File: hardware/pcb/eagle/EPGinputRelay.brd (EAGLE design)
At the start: 45 x 22 mm, 28 parts, among them J1 54-00248, U1 ADA4530-1, U2 ADA4530-1, U3 ADA4940-1

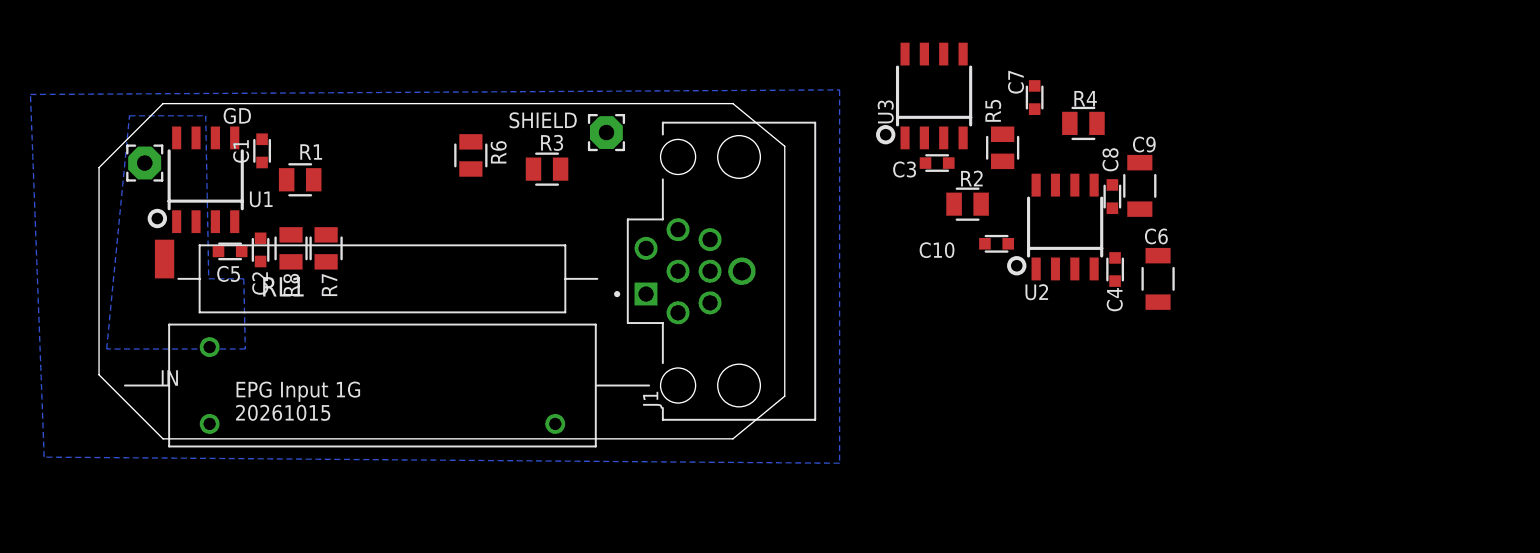
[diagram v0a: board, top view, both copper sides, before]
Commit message: PCB w/ relay
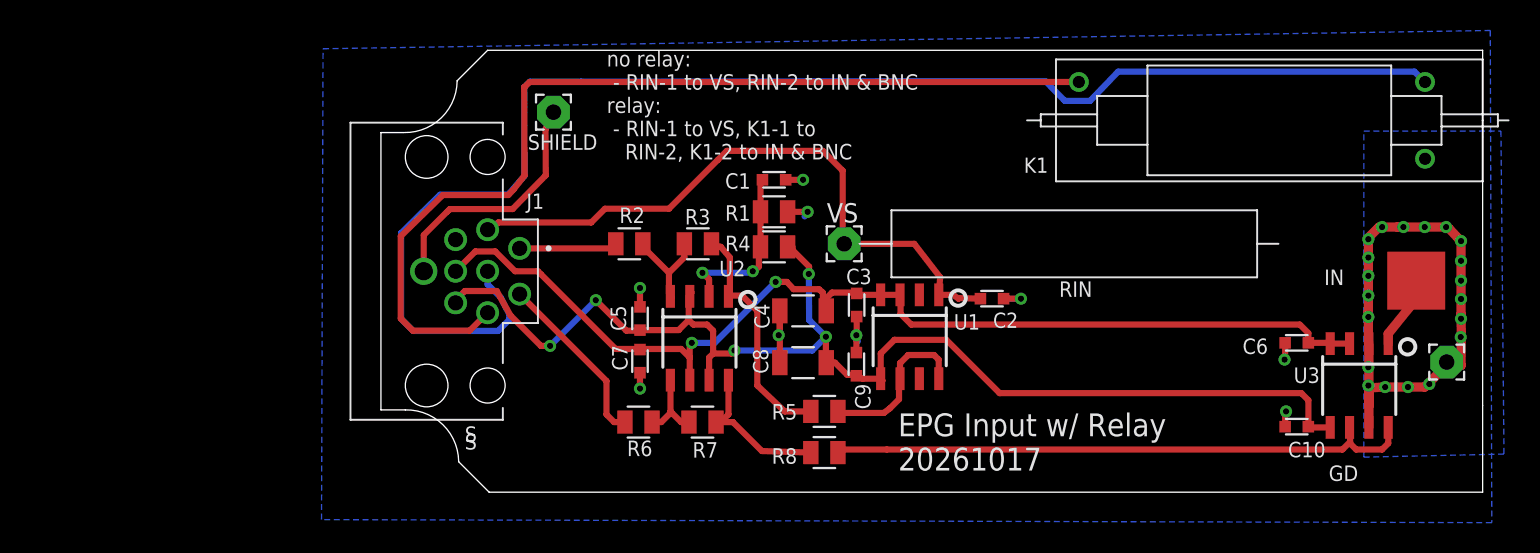
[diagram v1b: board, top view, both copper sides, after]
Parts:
- removed RL1: REED-RELAY, EPGinput:MRE05
- removed U$2: (no value), EPGinput:1GRES
- added K1: REED-RELAY, EPGinput:MRE05
- added RIN: (no value), EPGinput:1GRES
- added VS: (no value), wirepad:2,15/1,0
- C10: value 0.1 -> (none)
- C2: value (none) -> 0.1
- C4, C8: value (none) -> 10; device STEVES_BU:0603S -> STEVES_BU:1206S
- C6, C9: value 10 -> (none); device STEVES_BU:1206S -> STEVES_BU:0603S
- IN: device wirepad:SMD1,27-2,54 -> jETPAK-ASM:PAD-150SQ
- U$1: value POMONA2397 -> (none); device STEVES_BU:POMONA2397 -> EPGinput:BNC
- U2: value ADA4530-1 -> ADA4940-1
- U3: value ADA4940-1 -> ADA4530-1
- moved GD 86.4 mm to (69.9, -5.96), turned to 180 degrees
- moved IN 82.2 mm to (67.9, -0.62)
- moved C2 48.1 mm to (40.1, -1.80), turned to 0 degrees
- moved U$1 48.0 mm to (83.8, 0.00)
- moved U1 47.3 mm to (34.7, -4.30), turned to 180 degrees
- moved R8 37.5 mm to (29.1, -11.9), turned to 180 degrees
- moved U3 33.8 mm to (64.2, -7.50), turned to 180 degrees
- moved C1 33.7 mm to (25.8, 6.00), turned to 0 degrees
- moved R1 31.2 mm to (25.8, 3.90), turned to 180 degrees
- moved C7 31.1 mm to (17.0, -5.90)
- moved C5 27.3 mm to (17.0, -3.10), turned to 90 degrees
- moved R7 27.2 mm to (21.1, -9.90), turned to 180 degrees
- moved U2 25.1 mm to (20.9, -4.40), turned to 180 degrees
- moved C10 23.1 mm to (60.1, -10.2)
- moved C8 23.0 mm to (27.7, -6.00), turned to 180 degrees
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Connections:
- removed net N$1: C2.1, R7.1, R8.2, U3.2
- removed net RLY: J1.3, RL1.COIL2
- removed net SHIELD: J1.8, J1.S1, SHIELD.1
- new net N$2: J1.S1, SHIELD.1
- new net RLY+: J1.3, K1.COIL2
- new net RLY-: J1.8, K1.COIL1
- new net VCOM: C1.1, R1.2, R4.1, U2.2
- net -5V0: now also C3.1, U2.6, U3.3, U3.4; no longer C5.1, U2.3, U2.4, U3.6
- net 5V0: now also C10.1, C5.1, C8.1, C9.2, R4.2, U2.3, U2.7, U3.5; no longer C1.1, C3.1, C8.2, C9.1, R7.2, U2.5, U3.3, U3.7
- net GND: now also C8.2, C9.1, R1.1; no longer C8.1, C9.2, R8.1, RL1.COIL1
- net GUARD: now also K1.GUARD, U3.2, U3.7; no longer RL1.GUARD, U1.2, U1.7
- net N$10: now also R2.2; no longer R4.2
- net N$19: now also R2.1, R3.2, U2.4; no longer R4.1, R5.2, U3.4
- net N$20: now also R6.1, R7.2, U2.5; no longer R3.1, R6.2, U3.5
- net N$6: now also R7.1, R8.2, U2.8; no longer R1.2, R6.1, U3.8
- net N$7: now also R3.1, R5.2, U2.1; no longer R2.2, R5.1, U3.1
- net N$9: now also R6.2; no longer R3.2
- net PROBE: now also IN.P$1, U3.1; no longer IN.1, U1.1
- net SIGOUT: now also R8.1, U3.6, U3.8; no longer R1.1, U1.6, U1.8
- net VS: now also C2.1, U1.1, VS.1; no longer C10.1, U2.1
- net VSOUT: now also R5.1, U1.6, U1.8; no longer R2.1, U2.6, U2.8
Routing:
- net RLY-: track 0.00 -> 93.4 mm
- net 5V0: track 0.00 -> 83.0 mm, vias 0 -> 5
- net -5V0: track 0.00 -> 71.2 mm, vias 0 -> 2
- net RLY+: track 0.00 -> 64.1 mm
- net VS: track 0.00 -> 42.2 mm
- net SIGOUT: track 0.00 -> 38.8 mm
- net GUARD: track 0.00 -> 36.8 mm, vias 0 -> 20
- net GND: track 0.00 -> 18.6 mm, vias 0 -> 9
- net N$2: track 0.00 -> 16.3 mm
- net N$7: track 0.00 -> 15.4 mm
- net N$9: track 0.00 -> 11.7 mm
- net VCOM: track 0.00 -> 11.6 mm, vias 0 -> 2
- net VSOUT: track 0.00 -> 10.9 mm
- net N$6: track 0.00 -> 9.97 mm
- net N$19: track 0.00 -> 6.58 mm
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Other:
- board size 45 x 22 mm -> 72.3 x 29 mm
- board text added: "EPG Input w/ Relay 20261017"
- board text added: "S"
- board text added: "no relay: - RIN-1 to VS, RIN-2 to IN & BNC relay: - RIN-1 to VS, K1-1 to RIN-2, K1-2 to IN & BNC"
- board text removed: "EPG Input 1G 20261015"

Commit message: started control board
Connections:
- net N$10 renamed AOP\
- net N$9 renamed AON
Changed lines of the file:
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@@
 <layer number="14" name="Route14" color="1" fill="6" visible="no" active="no"/>
 <layer number="15" name="Route15" color="4" fill="6" visible="no" active="no"/>
-<layer number="16" name="Bottom" color="1" fill="1" visible="yes" active="yes"/>
+<layer number="16" name="Bottom" color="1" fill="1" visible="no" active="yes"/>
 <layer number="17" name="Pads" color="2" fill="1" visible="yes" active="yes"/>
 <layer number="18" name="Vias" color="2" fill="1" visible="yes" active="yes"/>
@@
 <layer number="20" name="Dimension" color="15" fill="1" visible="yes" active="yes"/>
 <layer number="21" name="tPlace" color="7" fill="1" visible="yes" active="yes"/>
-<layer number="22" name="bPlace" color="7" fill="1" visible="yes" active="yes"/>
+<layer number="22" name="bPlace" color="7" fill="1" visible="no" active="yes"/>
 <layer number="23" name="tOrigins" color="15" fill="1" visible="yes" active="yes"/>
-<layer number="24" name="bOrigins" color="15" fill="1" visible="yes" active="yes"/>
+<layer number="24" name="bOrigins" color="15" fill="1" visible="no" active="yes"/>
 <layer number="25" name="tNames" color="7" fill="1" visible="yes" active="yes"/>
-<layer number="26" name="bNames" color="7" fill="1" visible="yes" active="yes"/>
+<layer number="26" name="bNames" color="7" fill="1" visible="no" active="yes"/>
 <layer number="27" name="tValues" color="7" fill="1" visible="no" active="yes"/>
 <layer number="28" name="bValues" color="7" fill="1" visible="no" active="yes"/>
@@
 <via x="64.8" y="2.1" extent="1-16" drill="0.4"/>
 </signal>
-<signal name="N$9">
+<signal name="AON">
 <contactref element="R6" pad="2"/>
 <contactref element="J1" pad="2"/>
@@
 <wire x1="14.8" y1="-7.2" x2="9.1" y2="-1.5" width="0.4064" layer="1"/>
 </signal>
-<signal name="N$10">
+<signal name="AOP\">
 <contactref element="R2" pad="2"/>
 <contactref element="J1" pad="1"/>
